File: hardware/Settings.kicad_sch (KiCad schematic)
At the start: 9 parts, among them Q2 2N7002

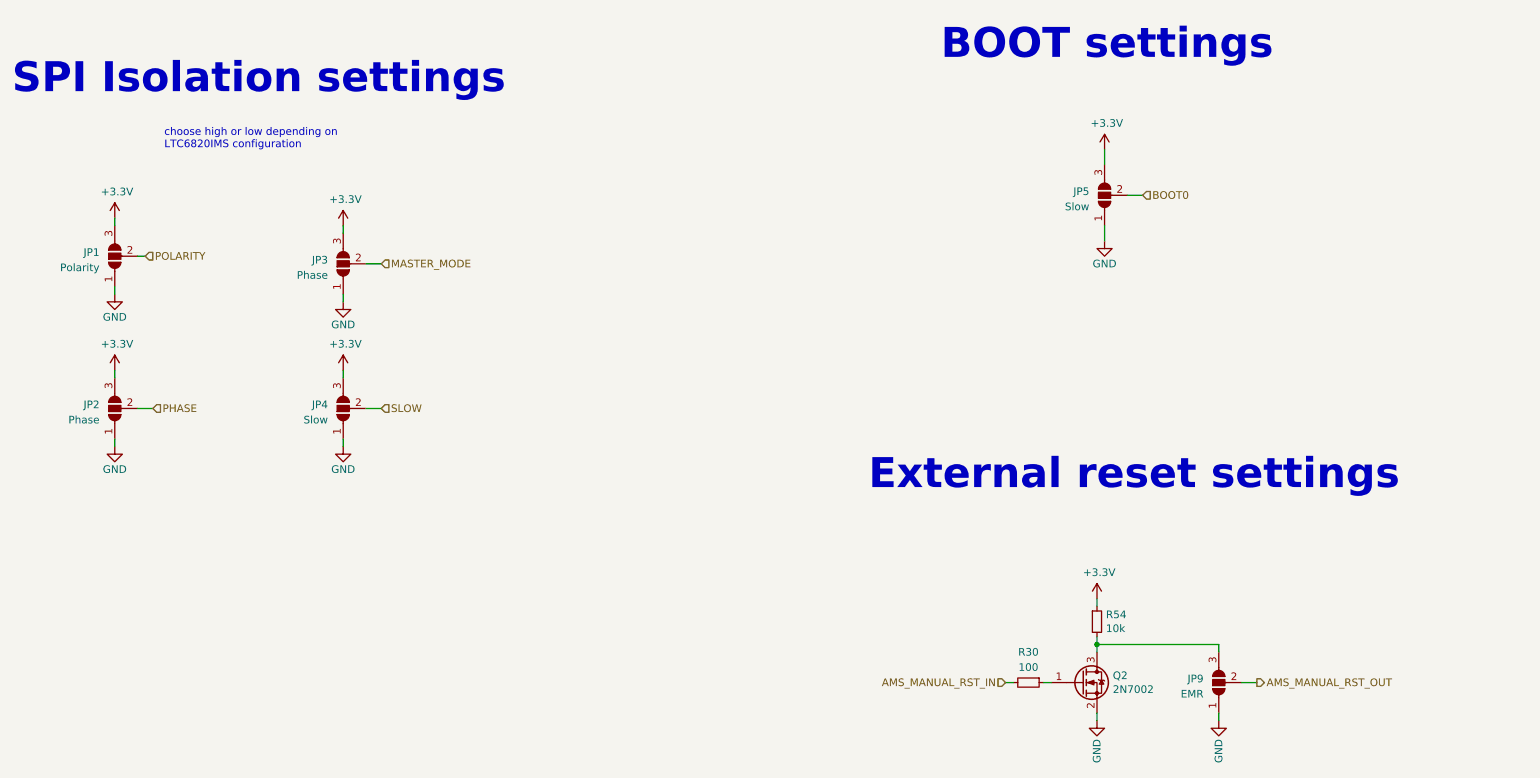
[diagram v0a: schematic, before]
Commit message: done
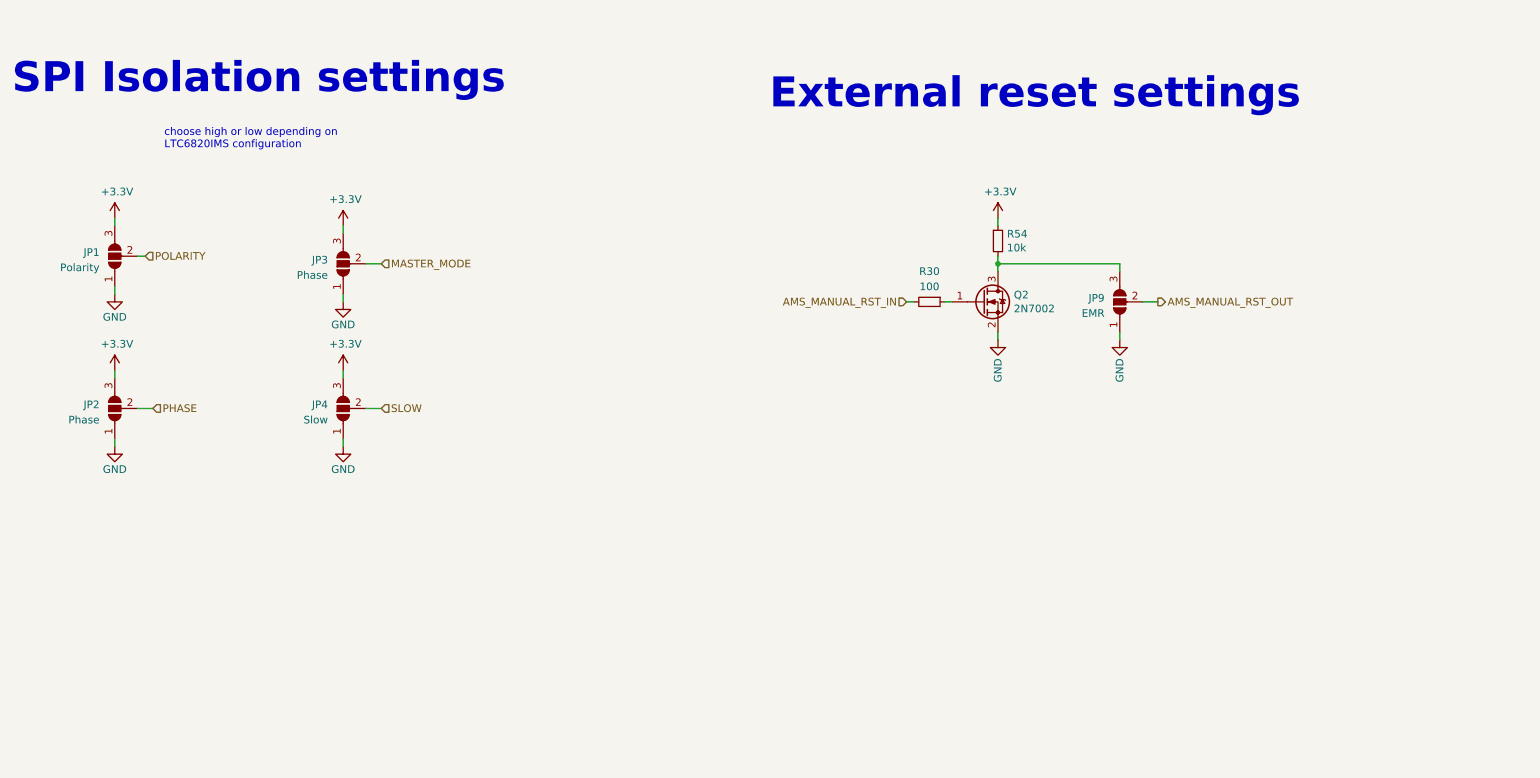
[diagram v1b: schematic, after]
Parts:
- removed JP5: Slow, Jumper:SolderJumper-3_P2.0mm_Open_TrianglePad1.0x1.5mm_NumberLabels, symbol Jumper:SolderJumper_3_Open
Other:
- note removed: "BOOT settings"
- moved on the sheet: JP9, Q2, R30, R54
